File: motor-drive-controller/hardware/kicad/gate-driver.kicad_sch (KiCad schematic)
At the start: 12 parts, among them U3 DRV83053PHP

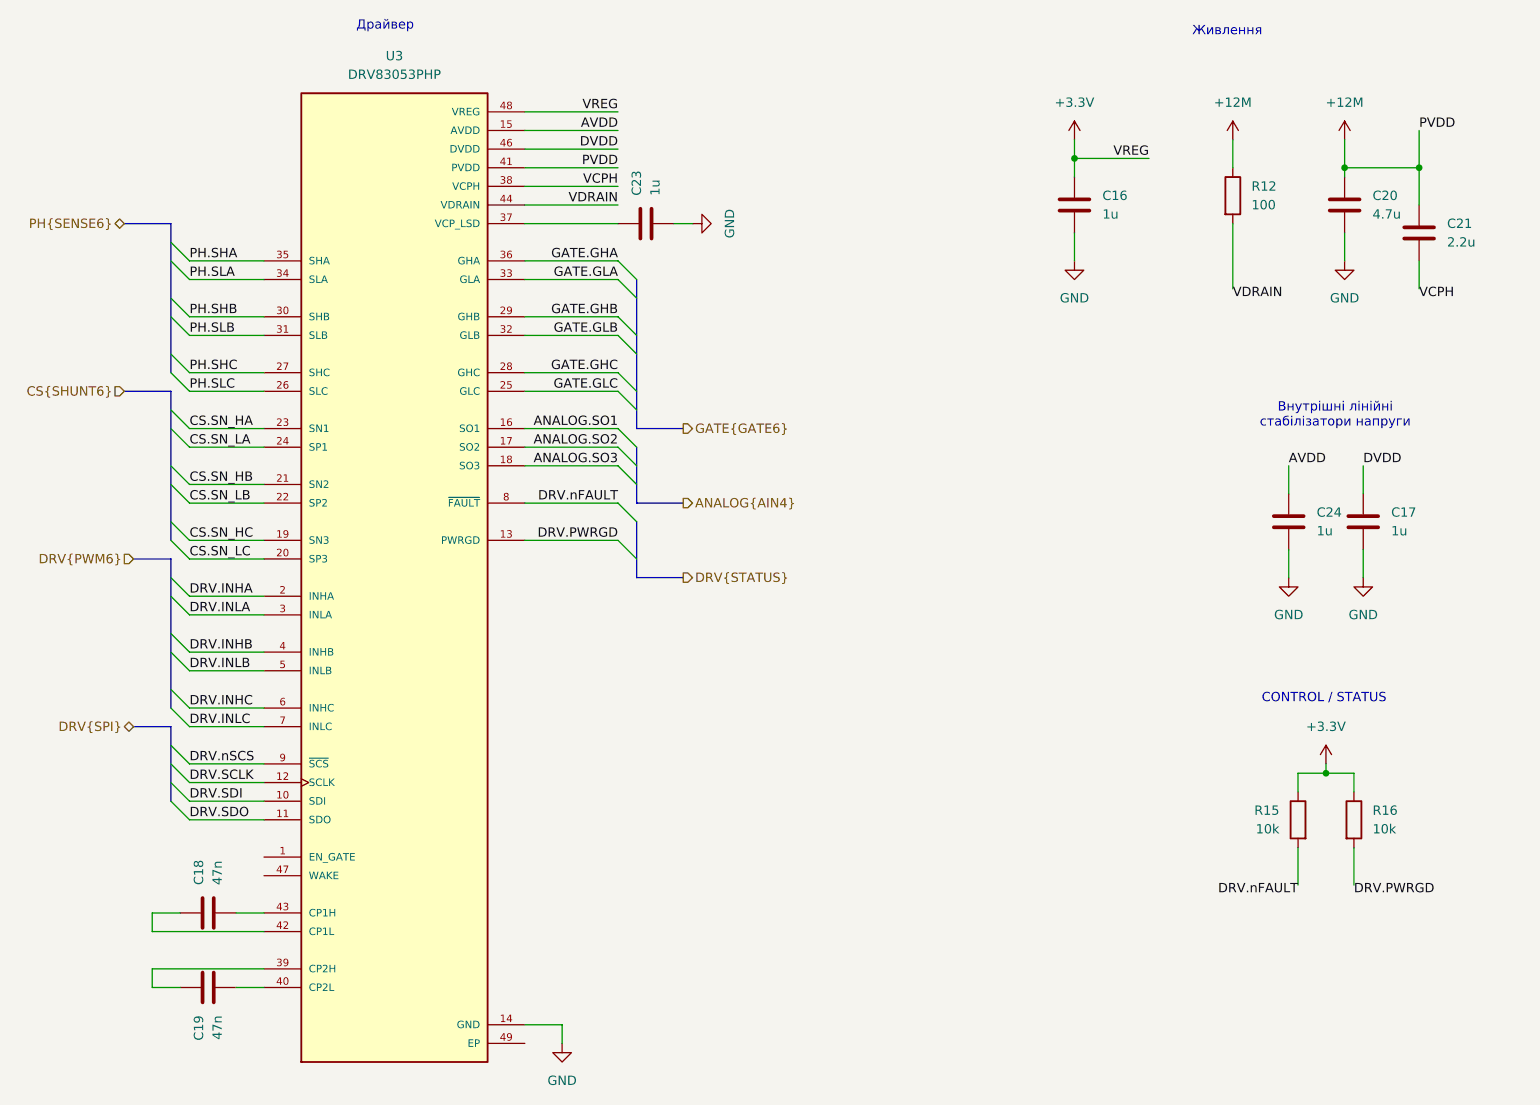
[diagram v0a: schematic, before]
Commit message: fix(hw09): fix ERC issues
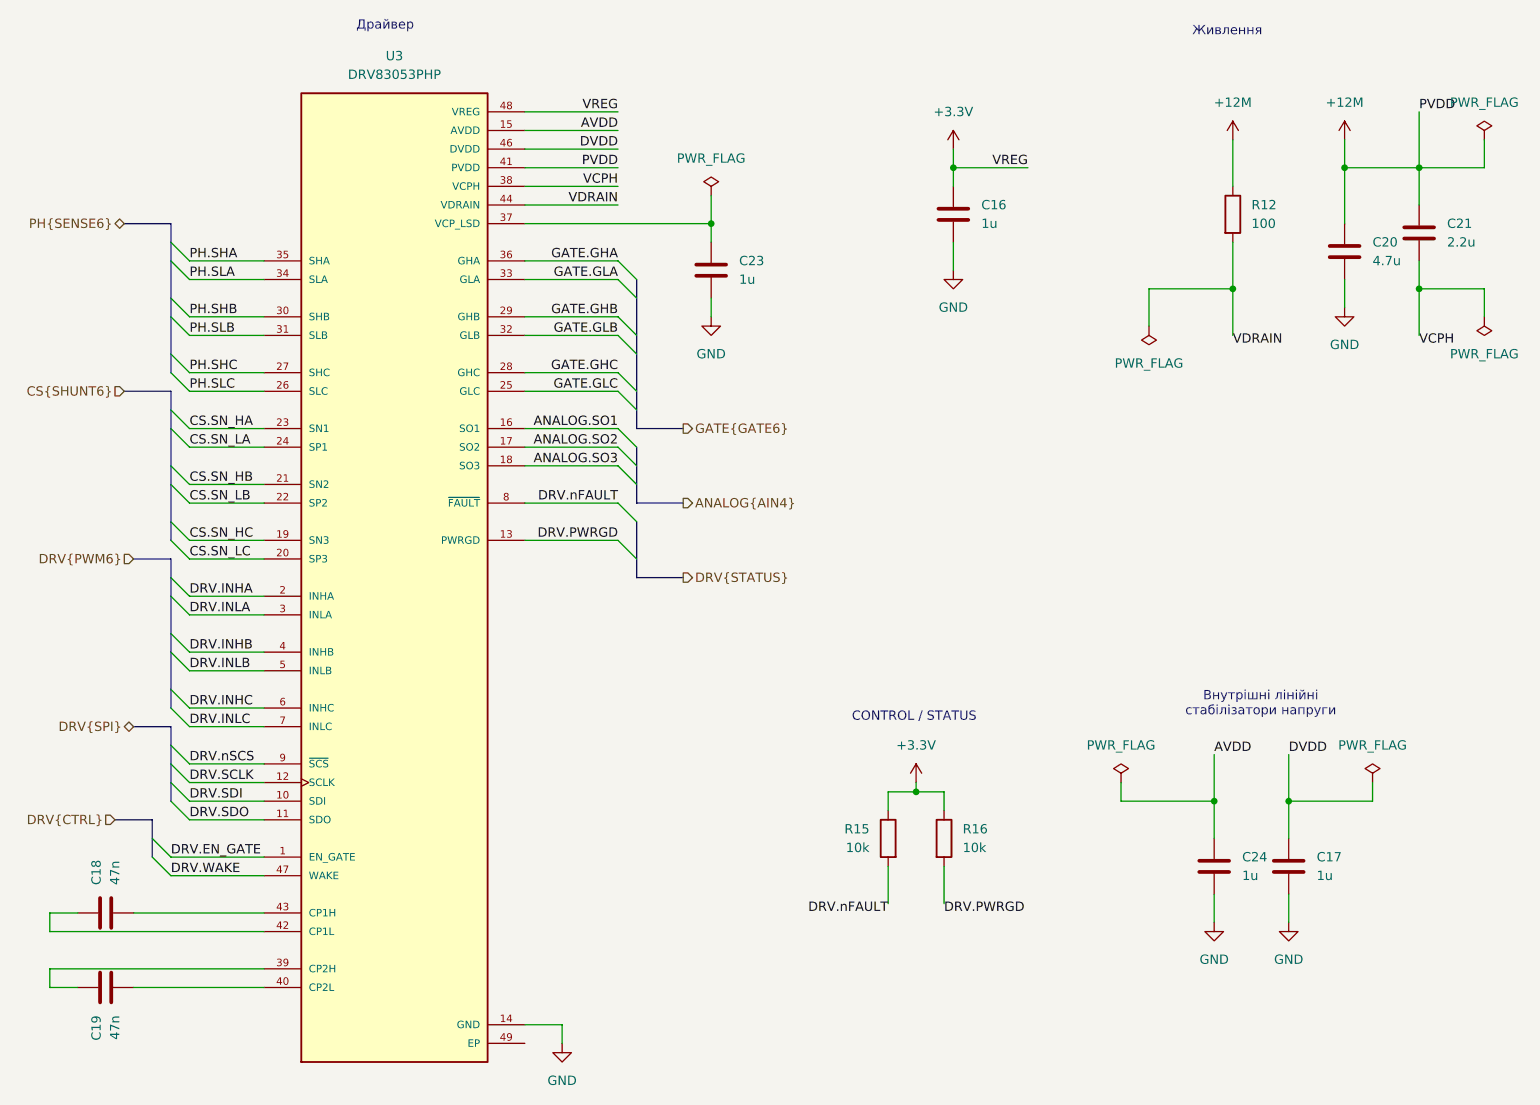
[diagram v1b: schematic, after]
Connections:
- net DRV.EN_GATE: now reaches U3.1 (EN_GATE)
- net DRV.WAKE: now reaches U3.47 (WAKE)
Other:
- moved on the sheet: C16, C17, C18, C19, C20, C23, C24, R12, R15, R16
